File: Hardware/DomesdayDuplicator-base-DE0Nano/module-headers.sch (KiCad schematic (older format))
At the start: 12 parts, among them J401 MOD0 Back, J402 MOD1 Back, J403 MOD0 Front, J404 MOD1 Front

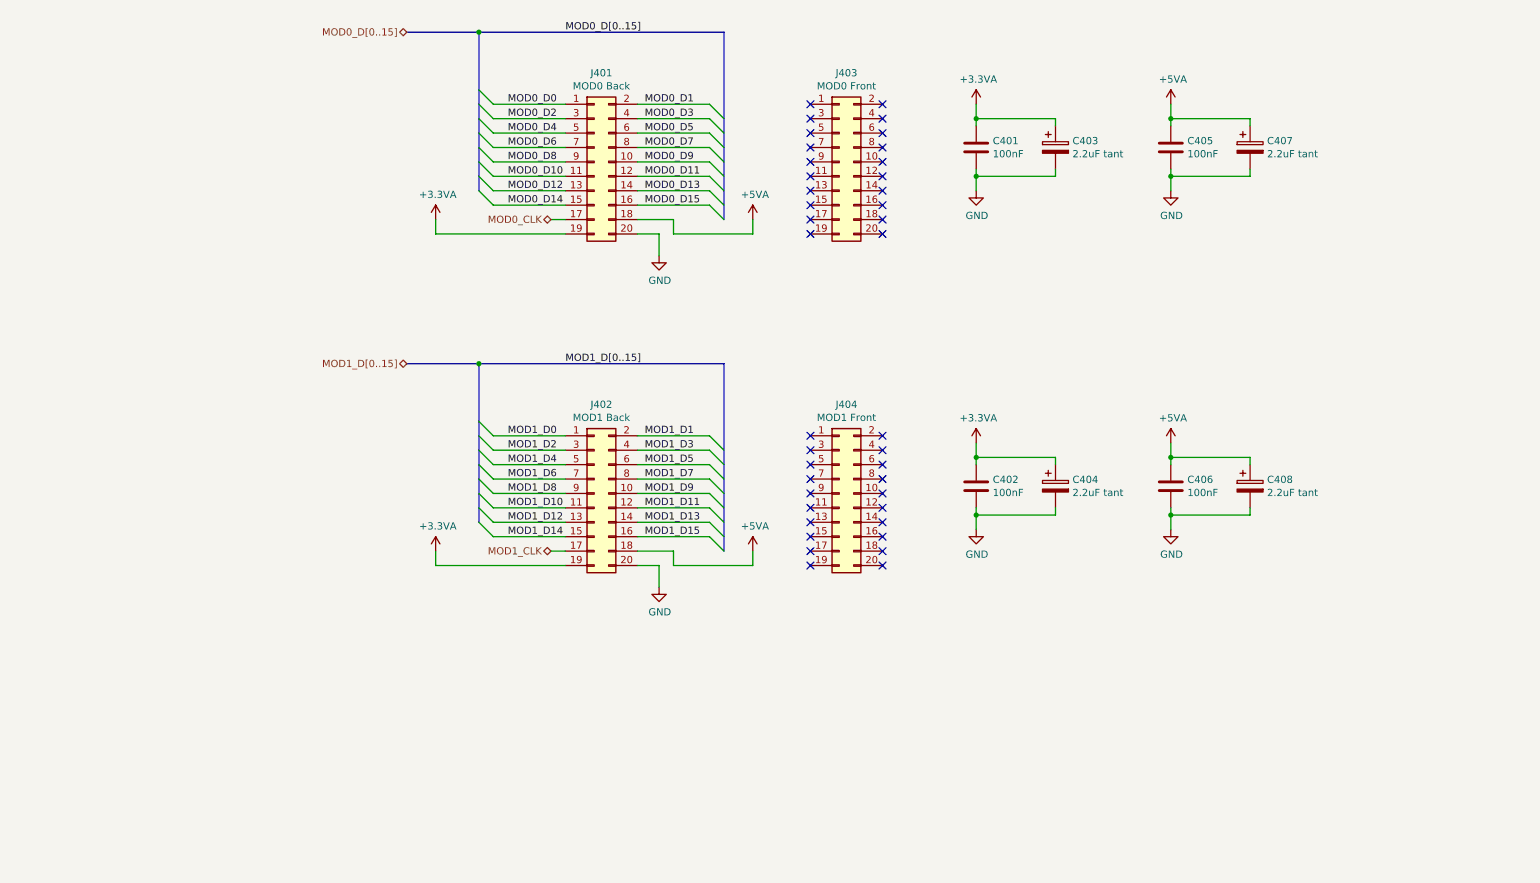
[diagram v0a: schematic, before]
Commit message: Added protection resistors to module headers on the base-board
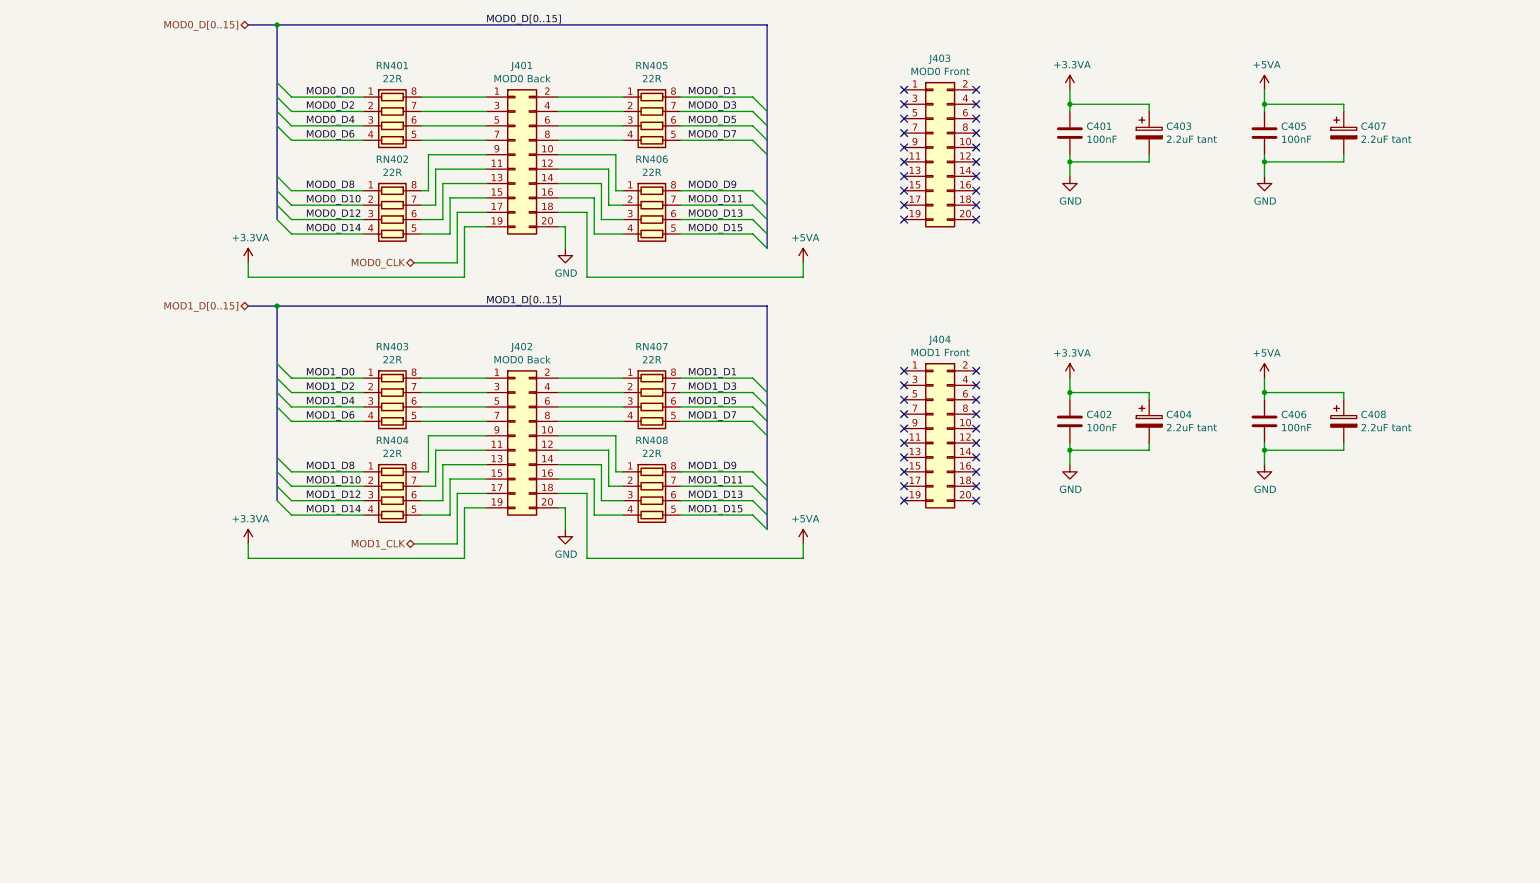
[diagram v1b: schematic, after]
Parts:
- added RN401, RN402, RN403, RN404, RN405, RN406, RN407, RN408: 22R, symbol Device:R_Pack04
- J402: value MOD1 Back -> MOD0 Back
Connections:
- net MOD0_D0: now also RN401.1 (R1.1); no longer J401.1 (Pin_1)
- net MOD0_D1: now also RN405.8 (R1.2); no longer J401.2 (Pin_2)
- net MOD0_D10: now also RN402.2 (R2.1); no longer J401.11 (Pin_11)
- net MOD0_D11: now also RN406.7 (R2.2); no longer J401.12 (Pin_12)
- net MOD0_D12: now also RN402.3 (R3.1); no longer J401.13 (Pin_13)
- net MOD0_D13: now also RN406.6 (R3.2); no longer J401.14 (Pin_14)
- net MOD0_D14: now also RN402.4 (R4.1); no longer J401.15 (Pin_15)
- net MOD0_D15: now also RN406.5 (R4.2); no longer J401.16 (Pin_16)
- net MOD0_D2: now also RN401.2 (R2.1); no longer J401.3 (Pin_3)
- net MOD0_D3: now also RN405.7 (R2.2); no longer J401.4 (Pin_4)
- net MOD0_D4: now also RN401.3 (R3.1); no longer J401.5 (Pin_5)
- net MOD0_D5: now also RN405.6 (R3.2); no longer J401.6 (Pin_6)
- net MOD0_D6: now also RN401.4 (R4.1); no longer J401.7 (Pin_7)
- net MOD0_D7: now also RN405.5 (R4.2); no longer J401.8 (Pin_8)
- net MOD0_D8: now also RN402.1 (R1.1); no longer J401.9 (Pin_9)
- net MOD0_D9: now also RN406.8 (R1.2); no longer J401.10 (Pin_10)
- net MOD1_D0: now also RN403.1 (R1.1); no longer J402.1 (Pin_1)
- net MOD1_D1: now also RN407.8 (R1.2); no longer J402.2 (Pin_2)
- net MOD1_D10: now also RN404.2 (R2.1); no longer J402.11 (Pin_11)
- net MOD1_D11: now also RN408.7 (R2.2); no longer J402.12 (Pin_12)
- net MOD1_D12: now also RN404.3 (R3.1); no longer J402.13 (Pin_13)
- net MOD1_D13: now also RN408.6 (R3.2); no longer J402.14 (Pin_14)
- net MOD1_D14: now also RN404.4 (R4.1); no longer J402.15 (Pin_15)
- net MOD1_D15: now also RN408.5 (R4.2); no longer J402.16 (Pin_16)
- net MOD1_D2: now also RN403.2 (R2.1); no longer J402.3 (Pin_3)
- net MOD1_D3: now also RN407.7 (R2.2); no longer J402.4 (Pin_4)
- net MOD1_D4: now also RN403.3 (R3.1); no longer J402.5 (Pin_5)
- net MOD1_D5: now also RN407.6 (R3.2); no longer J402.6 (Pin_6)
- net MOD1_D6: now also RN403.4 (R4.1); no longer J402.7 (Pin_7)
- net MOD1_D7: now also RN407.5 (R4.2); no longer J402.8 (Pin_8)
- net MOD1_D8: now also RN404.1 (R1.1); no longer J402.9 (Pin_9)
- net MOD1_D9: now also RN408.8 (R1.2); no longer J402.10 (Pin_10)
- new net: J401.7 (Pin_7), RN401.5 (R4.2)
- new net: J401.5 (Pin_5), RN401.6 (R3.2)
- new net: J401.3 (Pin_3), RN401.7 (R2.2)
- new net: J401.1 (Pin_1), RN401.8 (R1.2)
- new net: J401.15 (Pin_15), RN402.5 (R4.2)
- new net: J401.13 (Pin_13), RN402.6 (R3.2)
- new net: J401.11 (Pin_11), RN402.7 (R2.2)
- new net: J401.9 (Pin_9), RN402.8 (R1.2)
- new net: J401.2 (Pin_2), RN405.1 (R1.1)
- new net: J401.4 (Pin_4), RN405.2 (R2.1)
- new net: J401.6 (Pin_6), RN405.3 (R3.1)
- new net: J401.8 (Pin_8), RN405.4 (R4.1)
- new net: J401.10 (Pin_10), RN406.1 (R1.1)
- new net: J401.12 (Pin_12), RN406.2 (R2.1)
- new net: J401.14 (Pin_14), RN406.3 (R3.1)
- new net: J401.16 (Pin_16), RN406.4 (R4.1)
- new net: J402.1 (Pin_1), RN403.8 (R1.2)
- new net: J402.10 (Pin_10), RN408.1 (R1.1)
- new net: J402.11 (Pin_11), RN404.7 (R2.2)
- new net: J402.12 (Pin_12), RN408.2 (R2.1)
- new net: J402.13 (Pin_13), RN404.6 (R3.2)
- new net: J402.14 (Pin_14), RN408.3 (R3.1)
- new net: J402.15 (Pin_15), RN404.5 (R4.2)
- new net: J402.16 (Pin_16), RN408.4 (R4.1)
- new net: J402.2 (Pin_2), RN407.1 (R1.1)
- new net: J402.3 (Pin_3), RN403.7 (R2.2)
- new net: J402.4 (Pin_4), RN407.2 (R2.1)
- new net: J402.5 (Pin_5), RN403.6 (R3.2)
- new net: J402.6 (Pin_6), RN407.3 (R3.1)
- new net: J402.7 (Pin_7), RN403.5 (R4.2)
- new net: J402.8 (Pin_8), RN407.4 (R4.1)
- new net: J402.9 (Pin_9), RN404.8 (R1.2)
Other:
- moved on the sheet: C401, C402, C403, C404, C405, C406, C407, C408, J401, J403, J404

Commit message: Work on the ADS825 module to determine the overall module dimensions and mounting
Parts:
- J401, J402, J403, J404: footprint Connector_PinSocket_1.27mm:PinSocket_2x10_P1.27mm_Vertical_SMD -> Connector_Hirose:Hirose_DF12_DF12C3.0-20DS-0.5V_2x10_P0.50mm_Vertical
- RN401, RN402, RN403, RN404, RN405, RN406, RN407, RN408: footprint (none) -> Resistor_SMD:R_Array_Convex_4x1206
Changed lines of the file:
@@
 F 0 "J401" H 4050 3367 50  0000 C CNN
 F 1 "MOD0 Back" H 4050 3276 50  0000 C CNN
-F 2 "Connector_PinSocket_1.27mm:PinSocket_2x10_P1.27mm_Vertical_SMD" H 4000 2750 50  0001 C CNN
+F 2 "Connector_Hirose:Hirose_DF12_DF12C3.0-20DS-0.5V_2x10_P0.50mm_Vertical" H 4000 2750 50  0001 C CNN
 F 3 "~" H 4000 2750 50  0001 C CNN
 	1    4000 2750
@@
 F 0 "J403" H 6950 3317 50  0000 C CNN
 F 1 "MOD0 Front" H 6950 3226 50  0000 C CNN
-F 2 "Connector_PinSocket_1.27mm:PinSocket_2x10_P1.27mm_Vertical_SMD" H 6900 2700 50  0001 C CNN
+F 2 "Connector_Hirose:Hirose_DF12_DF12C3.0-20DS-0.5V_2x10_P0.50mm_Vertical" H 6900 2700 50  0001 C CNN
 F 3 "~" H 6900 2700 50  0001 C CNN
 	1    6900 2700
@@
 F 0 "J404" H 6950 5267 50  0000 C CNN
 F 1 "MOD1 Front" H 6950 5176 50  0000 C CNN
-F 2 "Connector_PinSocket_1.27mm:PinSocket_2x10_P1.27mm_Vertical_SMD" H 6900 4650 50  0001 C CNN
+F 2 "Connector_Hirose:Hirose_DF12_DF12C3.0-20DS-0.5V_2x10_P0.50mm_Vertical" H 6900 4650 50  0001 C CNN
 F 3 "~" H 6900 4650 50  0001 C CNN
 	1    6900 4650
@@
 F 0 "RN401" V 2733 2550 50  0000 C CNN
 F 1 "22R" V 2824 2550 50  0000 C CNN
-F 2 "" V 3425 2550 50  0001 C CNN
+F 2 "Resistor_SMD:R_Array_Convex_4x1206" V 3425 2550 50  0001 C CNN
 F 3 "~" H 3150 2550 50  0001 C CNN
 	1    3150 2550
@@
 F 0 "RN402" V 2733 3200 50  0000 C CNN
 F 1 "22R" V 2824 3200 50  0000 C CNN
-F 2 "" V 3425 3200 50  0001 C CNN
+F 2 "Resistor_SMD:R_Array_Convex_4x1206" V 3425 3200 50  0001 C CNN
 F 3 "~" H 3150 3200 50  0001 C CNN
 	1    3150 3200
@@
 F 0 "RN405" V 4533 2550 50  0000 C CNN
 F 1 "22R" V 4624 2550 50  0000 C CNN
-F 2 "" V 5225 2550 50  0001 C CNN
+F 2 "Resistor_SMD:R_Array_Convex_4x1206" V 5225 2550 50  0001 C CNN
 F 3 "~" H 4950 2550 50  0001 C CNN
 	1    4950 2550
@@
 F 0 "RN406" V 4533 3200 50  0000 C CNN
 F 1 "22R" V 4624 3200 50  0000 C CNN
-F 2 "" V 5225 3200 50  0001 C CNN
+F 2 "Resistor_SMD:R_Array_Convex_4x1206" V 5225 3200 50  0001 C CNN
 F 3 "~" H 4950 3200 50  0001 C CNN
 	1    4950 3200
@@
 F 0 "J402" H 4050 5317 50  0000 C CNN
 F 1 "MOD0 Back" H 4050 5226 50  0000 C CNN
-F 2 "Connector_PinSocket_1.27mm:PinSocket_2x10_P1.27mm_Vertical_SMD" H 4000 4700 50  0001 C CNN
+F 2 "Connector_Hirose:Hirose_DF12_DF12C3.0-20DS-0.5V_2x10_P0.50mm_Vertical" H 4000 4700 50  0001 C CNN
 F 3 "~" H 4000 4700 50  0001 C CNN
 	1    4000 4700
@@
 F 0 "RN403" V 2733 4500 50  0000 C CNN
 F 1 "22R" V 2824 4500 50  0000 C CNN
-F 2 "" V 3425 4500 50  0001 C CNN
+F 2 "Resistor_SMD:R_Array_Convex_4x1206" V 3425 4500 50  0001 C CNN
 F 3 "~" H 3150 4500 50  0001 C CNN
 	1    3150 4500
@@
 F 0 "RN404" V 2733 5150 50  0000 C CNN
 F 1 "22R" V 2824 5150 50  0000 C CNN
-F 2 "" V 3425 5150 50  0001 C CNN
+F 2 "Resistor_SMD:R_Array_Convex_4x1206" V 3425 5150 50  0001 C CNN
 F 3 "~" H 3150 5150 50  0001 C CNN
 	1    3150 5150
@@
 F 0 "RN407" V 4533 4500 50  0000 C CNN
 F 1 "22R" V 4624 4500 50  0000 C CNN
-F 2 "" V 5225 4500 50  0001 C CNN
+F 2 "Resistor_SMD:R_Array_Convex_4x1206" V 5225 4500 50  0001 C CNN
 F 3 "~" H 4950 4500 50  0001 C CNN
 	1    4950 4500
@@
 F 0 "RN408" V 4533 5150 50  0000 C CNN
 F 1 "22R" V 4624 5150 50  0000 C CNN
-F 2 "" V 5225 5150 50  0001 C CNN
+F 2 "Resistor_SMD:R_Array_Convex_4x1206" V 5225 5150 50  0001 C CNN
 F 3 "~" H 4950 5150 50  0001 C CNN
 	1    4950 5150
